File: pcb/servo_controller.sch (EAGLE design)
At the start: 55 parts, among them IC1 PIC18F452, IC2 LM2936MP-3.0, IC3 MAX4173FESA+, Q1 10Mhz, U1 ARDUINOR3-DIMENSION

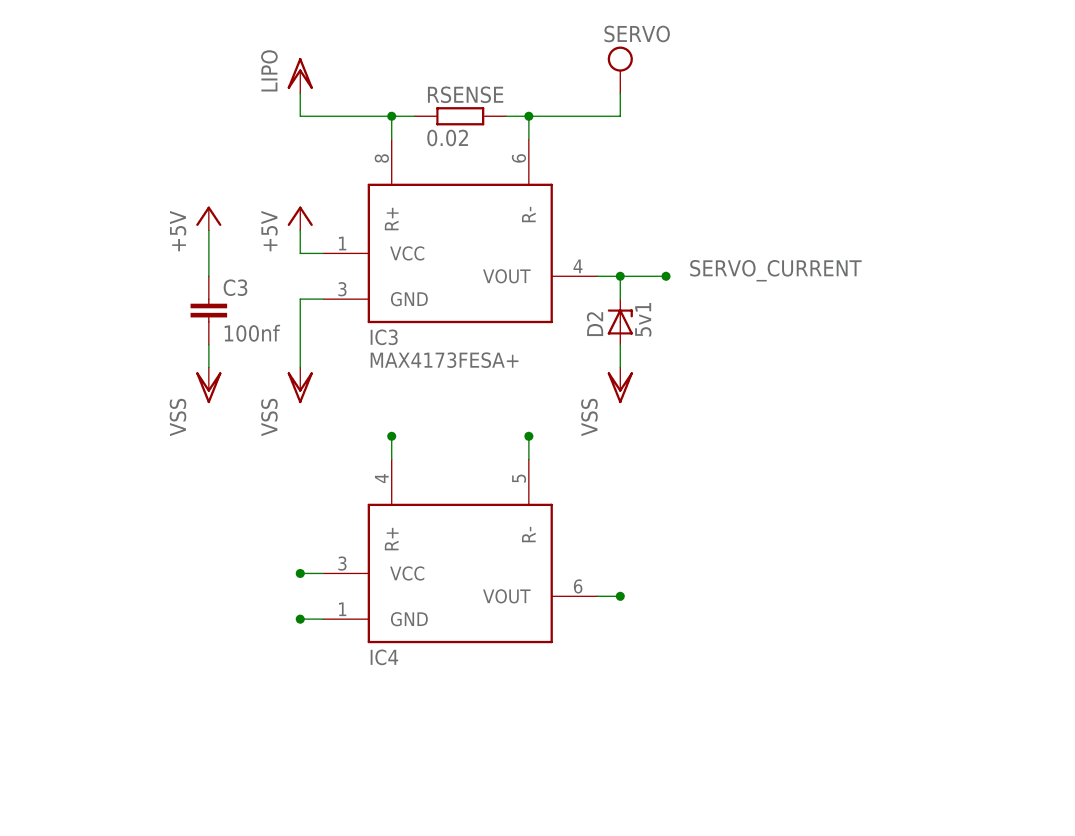
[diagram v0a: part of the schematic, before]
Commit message: Elec
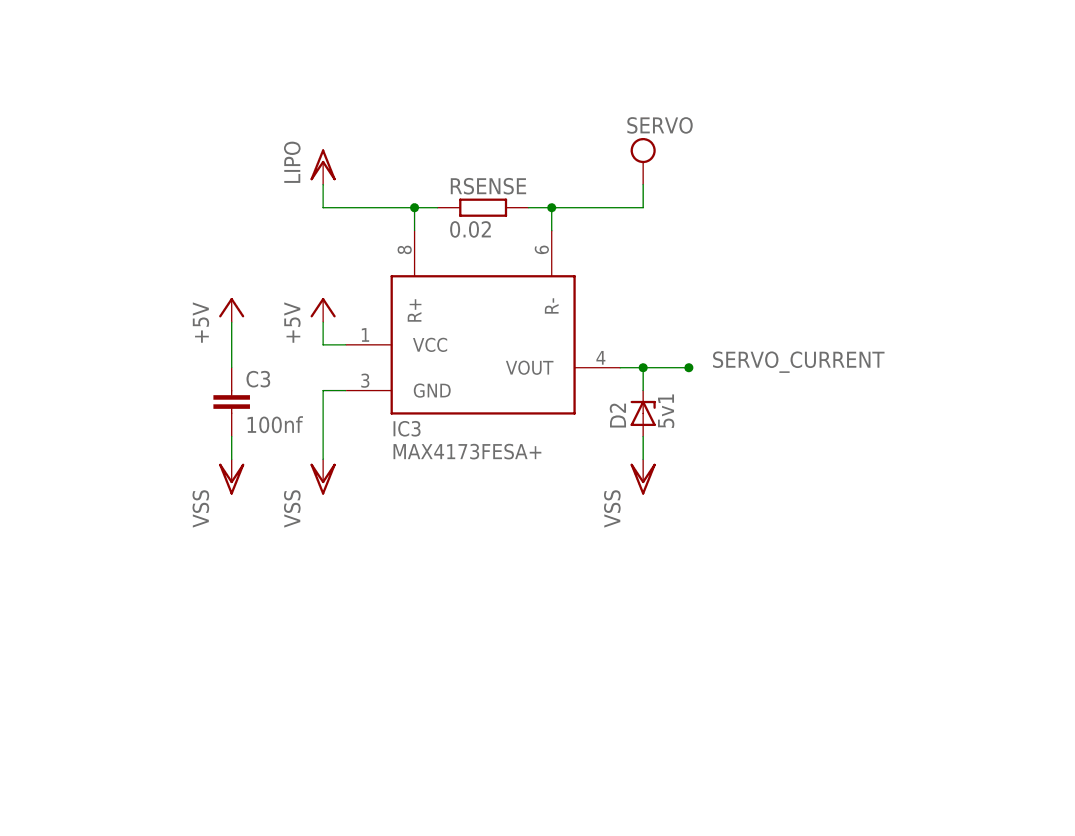
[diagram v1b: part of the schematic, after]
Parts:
- removed IC4: (no value), AWJLEagleLib:MAX4173T
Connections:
- net +5V: no longer IC4.VCC
- net SERVO_CURRENT: no longer IC4.VOUT
- net VDD: no longer IC4.R+
- net VEE: no longer IC4.R-
- net VSS: no longer IC4.GND
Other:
- moved on the sheet: C3, D2, IC3, RSENSE
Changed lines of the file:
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@@
 <part name="VSS27" library="supply1" deviceset="VSS" device=""/>
 <part name="PW" library="switch" deviceset="TL36PO" device=""/>
-<part name="IC4" library="AWJLEagleLib" deviceset="MAX4173" device="T"/>
 </parts>
 <sheets>
@@
 <instance part="VSS6" gate="G$1" x="48.26" y="177.8"/>
 <instance part="P+1" gate="1" x="121.92" y="215.9"/>
-<instance part="P+8" gate="1" x="195.58" y="215.9"/>
+<instance part="P+8" gate="1" x="198.12" y="205.74"/>
 <instance part="VSS7" gate="G$1" x="109.22" y="177.8"/>
 <instance part="VDD1" gate="G$1" x="48.26" y="215.9"/>
@@
 <instance part="SUPPLY3" gate="G$1" x="81.28" y="30.48"/>
 <instance part="SUPPLY4" gate="G$1" x="147.32" y="40.64"/>
-<instance part="IC3" gate="G$1" x="213.36" y="210.82"/>
-<instance part="VSS14" gate="G$1" x="195.58" y="195.58"/>
-<instance part="VDD2" gate="G$1" x="195.58" y="231.14"/>
+<instance part="IC3" gate="G$1" x="215.9" y="200.66"/>
+<instance part="VSS14" gate="G$1" x="198.12" y="185.42"/>
+<instance part="VDD2" gate="G$1" x="198.12" y="220.98"/>
 <instance part="RESET" gate="G$1" x="114.3" y="129.54" smashed="yes">
 <attribute name="NAME" x="114.935" y="130.81" size="1.778" layer="95" rot="R90"/>
@@
 <attribute name="TP_SIGNAL_NAME" x="125.73" y="128.27" size="1.778" layer="97"/>
 </instance>
-<instance part="SUPPLY5" gate="G$1" x="231.14" y="231.14"/>
+<instance part="SUPPLY5" gate="G$1" x="233.68" y="220.98"/>
 <instance part="VSS16" gate="G$1" x="134.62" y="101.6"/>
 <instance part="VSS17" gate="G$1" x="53.34" y="20.32"/>
@@
 </instance>
 <instance part="D1" gate="G$1" x="114.3" y="210.82"/>
-<instance part="C3" gate="G$1" x="185.42" y="205.74"/>
-<instance part="P+6" gate="1" x="185.42" y="215.9"/>
-<instance part="VSS8" gate="G$1" x="185.42" y="195.58"/>
+<instance part="C3" gate="G$1" x="187.96" y="195.58"/>
+<instance part="P+6" gate="1" x="187.96" y="205.74"/>
+<instance part="VSS8" gate="G$1" x="187.96" y="185.42"/>
 <instance part="EXT" gate="1" x="299.72" y="50.8"/>
 <instance part="C5" gate="G$1" x="60.96" y="30.48"/>
 <instance part="VSS22" gate="G$1" x="60.96" y="20.32"/>
-<instance part="RSENSE" gate="G$1" x="213.36" y="226.06"/>
+<instance part="RSENSE" gate="G$1" x="215.9" y="215.9"/>
 <instance part="C4" gate="G$1" x="182.88" y="27.94"/>
 <instance part="VSS23" gate="G$1" x="182.88" y="17.78"/>
@@
 <instance part="R7" gate="G$1" x="83.82" y="93.98" rot="R90"/>
 <instance part="P+9" gate="1" x="83.82" y="104.14"/>
-<instance part="D2" gate="G$1" x="231.14" y="203.2" rot="R90"/>
+<instance part="D2" gate="G$1" x="233.68" y="193.04" rot="R90"/>
 <instance part="D3" gate="G$1" x="55.88" y="187.96" rot="R90"/>
 <instance part="VSS25" gate="G$1" x="55.88" y="177.8"/>
-<instance part="VSS26" gate="G$1" x="231.14" y="195.58"/>
+<instance part="VSS26" gate="G$1" x="233.68" y="185.42"/>
 <instance part="SJ1" gate="1" x="332.74" y="129.54" rot="R90"/>
 <instance part="C9" gate="G$1" x="119.38" y="198.12"/>
 <instance part="VSS27" gate="G$1" x="119.38" y="177.8"/>
 <instance part="PW" gate="BEF1" x="35.56" y="208.28" rot="R270"/>
-<instance part="IC4" gate="G$1" x="213.36" y="175.26"/>
 </instances>
 <busses>
@@
 <segment>
 <pinref part="IC3" gate="G$1" pin="GND"/>
-<wire x1="198.12" y1="205.74" x2="195.58" y2="205.74" width="0.1524" layer="91"/>
+<wire x1="200.66" y1="195.58" x2="198.12" y2="195.58" width="0.1524" layer="91"/>
 <pinref part="VSS14" gate="G$1" pin="VSS"/>
-<wire x1="195.58" y1="205.74" x2="195.58" y2="198.12" width="0.1524" layer="91"/>
+<wire x1="198.12" y1="195.58" x2="198.12" y2="187.96" width="0.1524" layer="91"/>
 </segment>
 <segment>
@@
 <pinref part="C3" gate="G$1" pin="2"/>
 <pinref part="VSS8" gate="G$1" pin="VSS"/>
-<wire x1="185.42" y1="198.12" x2="185.42" y2="200.66" width="0.1524" layer="91"/>
+<wire x1="187.96" y1="187.96" x2="187.96" y2="190.5" width="0.1524" layer="91"/>
 </segment>
 <segment>
@@
 <pinref part="D2" gate="G$1" pin="A"/>
 <pinref part="VSS26" gate="G$1" pin="VSS"/>
-<wire x1="231.14" y1="198.12" x2="231.14" y2="200.66" width="0.1524" layer="91"/>
+<wire x1="233.68" y1="187.96" x2="233.68" y2="190.5" width="0.1524" layer="91"/>
 </segment>
 <segment>
@@
 <pinref part="VSS27" gate="G$1" pin="VSS"/>
 <wire x1="119.38" y1="180.34" x2="119.38" y2="193.04" width="0.1524" layer="91"/>
-</segment>
-<segment>
-<pinref part="IC4" gate="G$1" pin="GND"/>
-<wire x1="198.12" y1="170.18" x2="195.58" y2="170.18" width="0.1524" layer="91"/>
-<junction x="195.58" y="170.18"/>
 </segment>
 </net>
@@
 <segment>
 <pinref part="IC3" gate="G$1" pin="VCC"/>
-<wire x1="198.12" y1="210.82" x2="195.58" y2="210.82" width="0.1524" layer="91"/>
+<wire x1="200.66" y1="200.66" x2="198.12" y2="200.66" width="0.1524" layer="91"/>
 <pinref part="P+8" gate="1" pin="+5V"/>
-<wire x1="195.58" y1="210.82" x2="195.58" y2="213.36" width="0.1524" layer="91"/>
+<wire x1="198.12" y1="200.66" x2="198.12" y2="203.2" width="0.1524" layer="91"/>
 </segment>
 <segment>
 <pinref part="P+6" gate="1" pin="+5V"/>
 <pinref part="C3" gate="G$1" pin="1"/>
-<wire x1="185.42" y1="208.28" x2="185.42" y2="213.36" width="0.1524" layer="91"/>
+<wire x1="187.96" y1="198.12" x2="187.96" y2="203.2" width="0.1524" layer="91"/>
 </segment>
 <segment>
@@
 <pinref part="P+9" gate="1" pin="+5V"/>
 <wire x1="83.82" y1="101.6" x2="83.82" y2="99.06" width="0.1524" layer="91"/>
-</segment>
-<segment>
-<pinref part="IC4" gate="G$1" pin="VCC"/>
-<wire x1="198.12" y1="175.26" x2="195.58" y2="175.26" width="0.1524" layer="91"/>
-<junction x="195.58" y="175.26"/>
 </segment>
 </net>
@@
 <segment>
 <pinref part="VDD2" gate="G$1" pin="VDD"/>
-<wire x1="195.58" y1="228.6" x2="195.58" y2="226.06" width="0.1524" layer="91"/>
-<wire x1="195.58" y1="226.06" x2="205.74" y2="226.06" width="0.1524" layer="91"/>
+<wire x1="198.12" y1="218.44" x2="198.12" y2="215.9" width="0.1524" layer="91"/>
+<wire x1="198.12" y1="215.9" x2="208.28" y2="215.9" width="0.1524" layer="91"/>
 <pinref part="IC3" gate="G$1" pin="R+"/>
-<wire x1="205.74" y1="226.06" x2="205.74" y2="223.52" width="0.1524" layer="91"/>
-<wire x1="205.74" y1="226.06" x2="208.28" y2="226.06" width="0.1524" layer="91"/>
-<junction x="205.74" y="226.06"/>
+<wire x1="208.28" y1="215.9" x2="208.28" y2="213.36" width="0.1524" layer="91"/>
+<wire x1="208.28" y1="215.9" x2="210.82" y2="215.9" width="0.1524" layer="91"/>
+<junction x="208.28" y="215.9"/>
 <pinref part="RSENSE" gate="G$1" pin="1"/>
-</segment>
-<segment>
-<pinref part="IC4" gate="G$1" pin="R+"/>
-<wire x1="205.74" y1="187.96" x2="205.74" y2="190.5" width="0.1524" layer="91"/>
-<junction x="205.74" y="190.5"/>
 </segment>
 </net>
@@
 <segment>
 <pinref part="IC3" gate="G$1" pin="R-"/>
-<wire x1="220.98" y1="223.52" x2="220.98" y2="226.06" width="0.1524" layer="91"/>
-<wire x1="220.98" y1="226.06" x2="231.14" y2="226.06" width="0.1524" layer="91"/>
+<wire x1="223.52" y1="213.36" x2="223.52" y2="215.9" width="0.1524" layer="91"/>
+<wire x1="223.52" y1="215.9" x2="233.68" y2="215.9" width="0.1524" layer="91"/>
 <pinref part="SUPPLY5" gate="G$1" pin="VEE"/>
-<wire x1="231.14" y1="226.06" x2="231.14" y2="228.6" width="0.1524" layer="91"/>
-<wire x1="218.44" y1="226.06" x2="220.98" y2="226.06" width="0.1524" layer="91"/>
-<junction x="220.98" y="226.06"/>
+<wire x1="233.68" y1="215.9" x2="233.68" y2="218.44" width="0.1524" layer="91"/>
+<wire x1="220.98" y1="215.9" x2="223.52" y2="215.9" width="0.1524" layer="91"/>
+<junction x="223.52" y="215.9"/>
 <pinref part="RSENSE" gate="G$1" pin="2"/>
 </segment>
-<segment>
-<pinref part="IC4" gate="G$1" pin="R-"/>
-<wire x1="220.98" y1="187.96" x2="220.98" y2="190.5" width="0.1524" layer="91"/>
-<junction x="220.98" y="190.5"/>
-</segment>
 </net>
 <net name="SERVO_CURRENT" class="0">
 <segment>
 <pinref part="IC3" gate="G$1" pin="VOUT"/>
-<wire x1="228.6" y1="208.28" x2="231.14" y2="208.28" width="0.1524" layer="91"/>
-<junction x="236.22" y="208.28"/>
-<label x="238.76" y="208.28" size="1.778" layer="95"/>
+<wire x1="231.14" y1="198.12" x2="233.68" y2="198.12" width="0.1524" layer="91"/>
+<junction x="238.76" y="198.12"/>
+<label x="241.3" y="198.12" size="1.778" layer="95"/>
 <pinref part="D2" gate="G$1" pin="C"/>
-<wire x1="231.14" y1="208.28" x2="236.22" y2="208.28" width="0.1524" layer="91"/>
-<wire x1="231.14" y1="208.28" x2="231.14" y2="205.74" width="0.1524" layer="91"/>
-<junction x="231.14" y="208.28"/>
+<wire x1="233.68" y1="198.12" x2="238.76" y2="198.12" width="0.1524" layer="91"/>
+<wire x1="233.68" y1="198.12" x2="233.68" y2="195.58" width="0.1524" layer="91"/>
+<junction x="233.68" y="198.12"/>
 </segment>
 <segment>
@@
 <label x="353.06" y="116.84" size="1.778" layer="95" rot="R90"/>
 </segment>
-<segment>
-<pinref part="IC4" gate="G$1" pin="VOUT"/>
-<wire x1="228.6" y1="172.72" x2="231.14" y2="172.72" width="0.1524" layer="91"/>
-<junction x="231.14" y="172.72"/>
-</segment>
-</net>
+</net>
